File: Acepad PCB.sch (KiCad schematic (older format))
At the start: 58 parts, among them SW1 SW_Push, U1 ATmega32U4-AU, Y1 16MHz

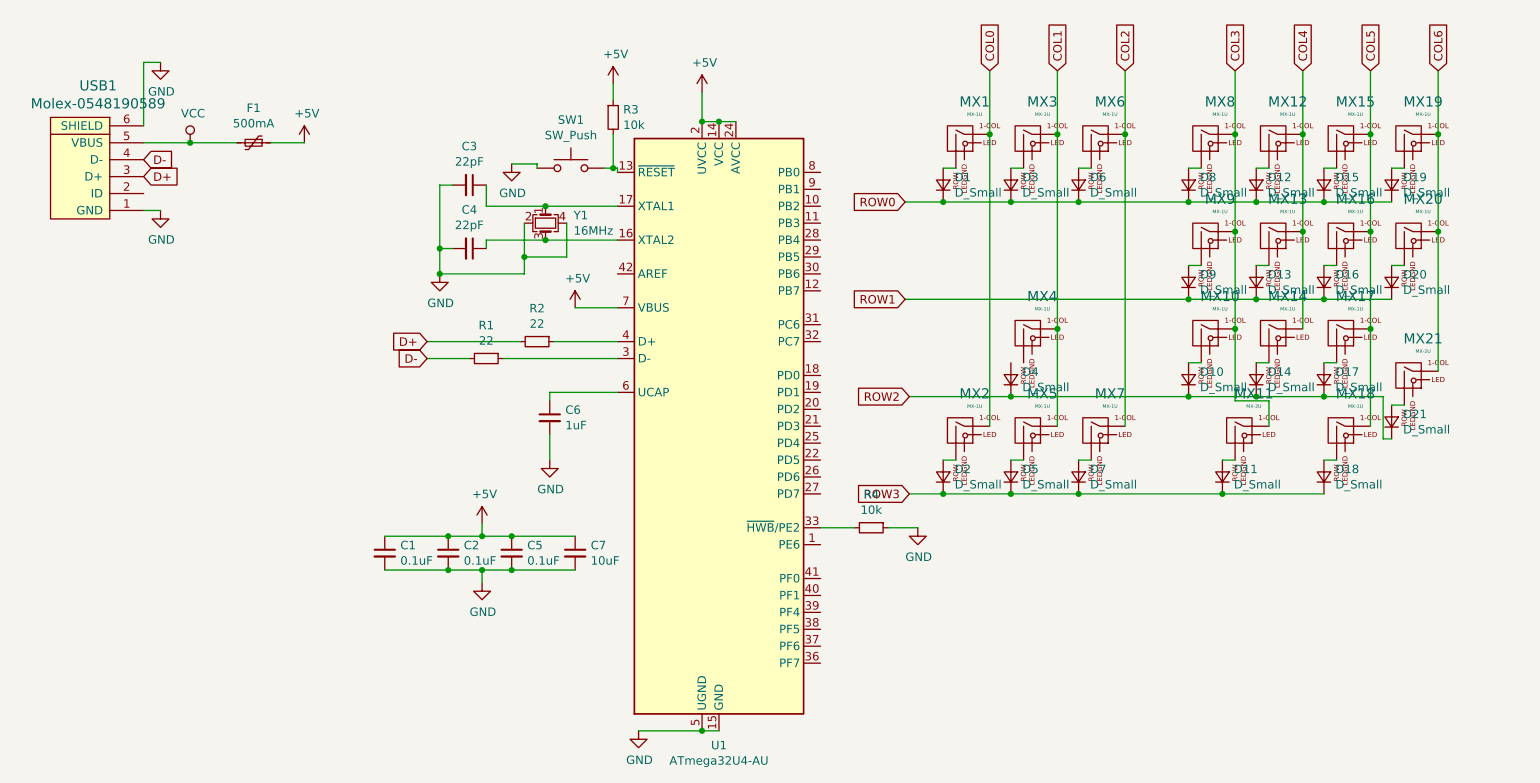
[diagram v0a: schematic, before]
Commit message: worked more on PCB
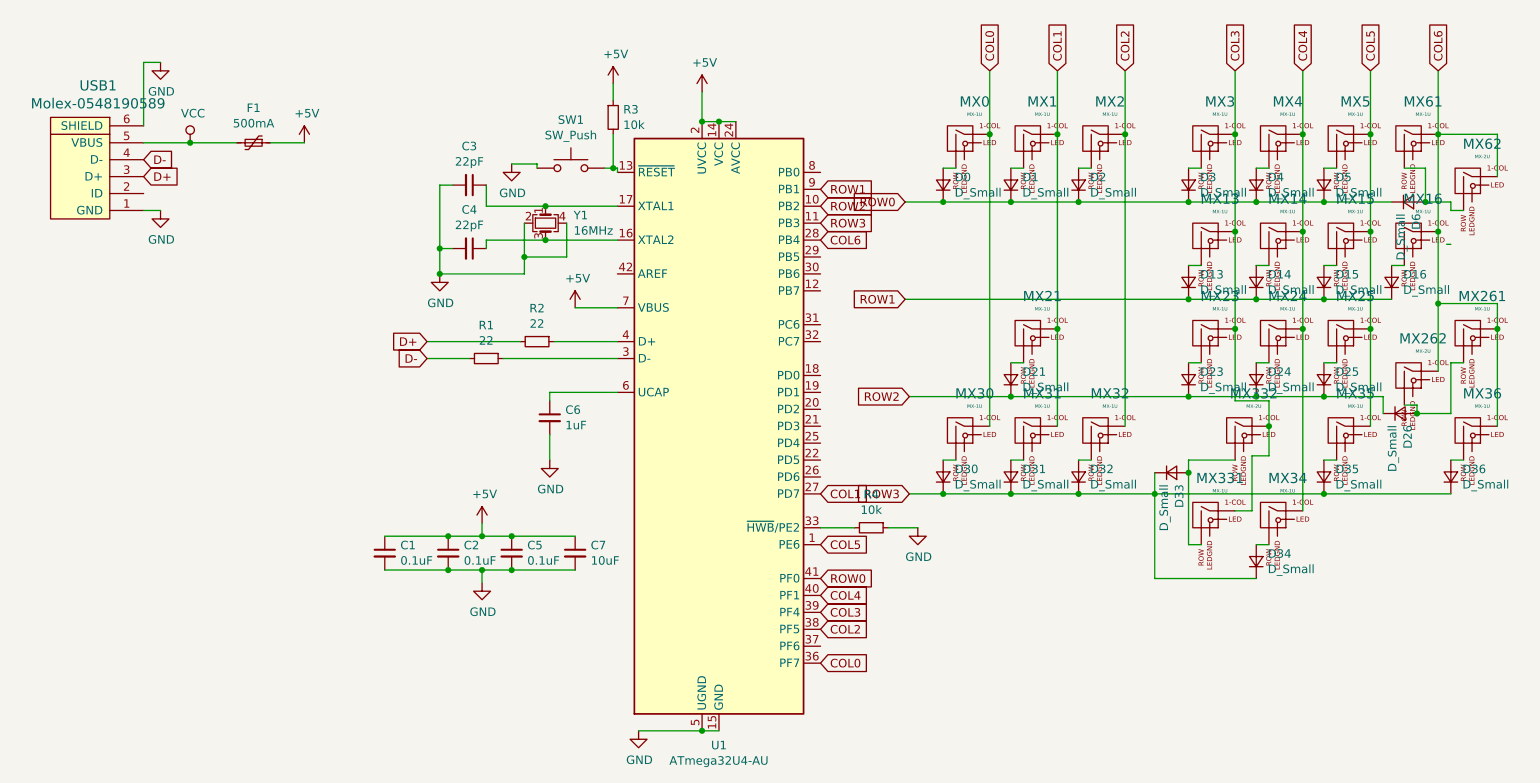
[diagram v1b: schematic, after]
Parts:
- removed D11: D_Small, Diode_SMD:D_SOD-123, symbol Device:D_Small
- added D33, D34, D36: D_Small, Diode_SMD:D_SOD-123, symbol Device:D_Small
- added MX261, MX331, MX34, MX36: MX-1U, MX_Alps_Hybrid:MX-1U, symbol MX_Alps_Hybrids:MX-1U
- added MX62: MX-2U, MX_Alps_Hybrid:MX-2U, symbol MX_Alps_Hybrids:MX-2U
- F1: footprint Housings_QFP:TQFP-44_10x10mm_Pitch0.8mm -> Fuse_Holders_and_Fuses:Fuse_SMD1206_Reflow
- renumbered D1 to D0, D3 to D1, D9 to D13, D13 to D14, D16 to D15, D20 to D16, D6 to D2, D4 to D21, D10 to D23, D14 to D24, D17 to D25, D21 to D26, D8 to D3, D2 to D30, D5 to D31, D7 to D32, D18 to D35, D12 to D4, D15 to D5, D19 to D6, MX1 to MX0, MX3 to MX1, MX9 to MX13, MX13 to MX14, MX16 to MX15, MX20 to MX16, MX6 to MX2, MX4 to MX21, MX10 to MX23, MX14 to MX24, MX17 to MX25, MX21 to MX262, MX8 to MX3, MX2 to MX30, MX5 to MX31, MX7 to MX32, MX11 to MX332, MX18 to MX35, MX12 to MX4, MX15 to MX5, MX19 to MX61
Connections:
- net COL0: now also U1.36 (PF7)
- net COL1: now also U1.27 (PD7)
- net COL2: now also U1.38 (PF5)
- net COL3: now also U1.39 (PF4), MX331.1 (COL)
- net COL4: now also U1.40 (PF1), MX34.1 (COL)
- net COL5: now also U1.1 (PE6)
- net COL6: now also U1.28 (PB4), MX261.1 (COL), MX36.1 (COL), MX62.1 (COL)
- net ROW0: now also U1.41 (PF0)
- net ROW1: now also U1.9 (PB1)
- net ROW2: now also U1.10 (PB2)
- net ROW3: now also U1.11 (PB3), D33.1 (K), D34.1 (K), D36.1 (K)
- net at MX21.2 (ROW): now also D21.2 (A)
- net at D6.2 (A), MX61.2 (ROW): now also MX62.2 (ROW)
- net at MX332.2 (ROW): now also D33.2 (A), MX331.2 (ROW)
- net at D26.2 (A), MX262.2 (ROW): now also MX261.2 (ROW)
- new net: D36.2 (A), MX36.2 (ROW)
- new net: D34.2 (A), MX34.2 (ROW)
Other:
- moved on the sheet: D26, D6
